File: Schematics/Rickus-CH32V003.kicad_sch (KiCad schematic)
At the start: 31 parts, among them J1 USB_C_Receptacle_USB2.0, J3 Conn_01x03, J4 OledDisplay, J6 uSD Card, SW2 Power, SW2 SW_MEC_5E, U1 CH32V003f4p6, U1 CH340E, U2 8 megabytes SPI PSRAM, U3 LD1117S12TR_SOT223

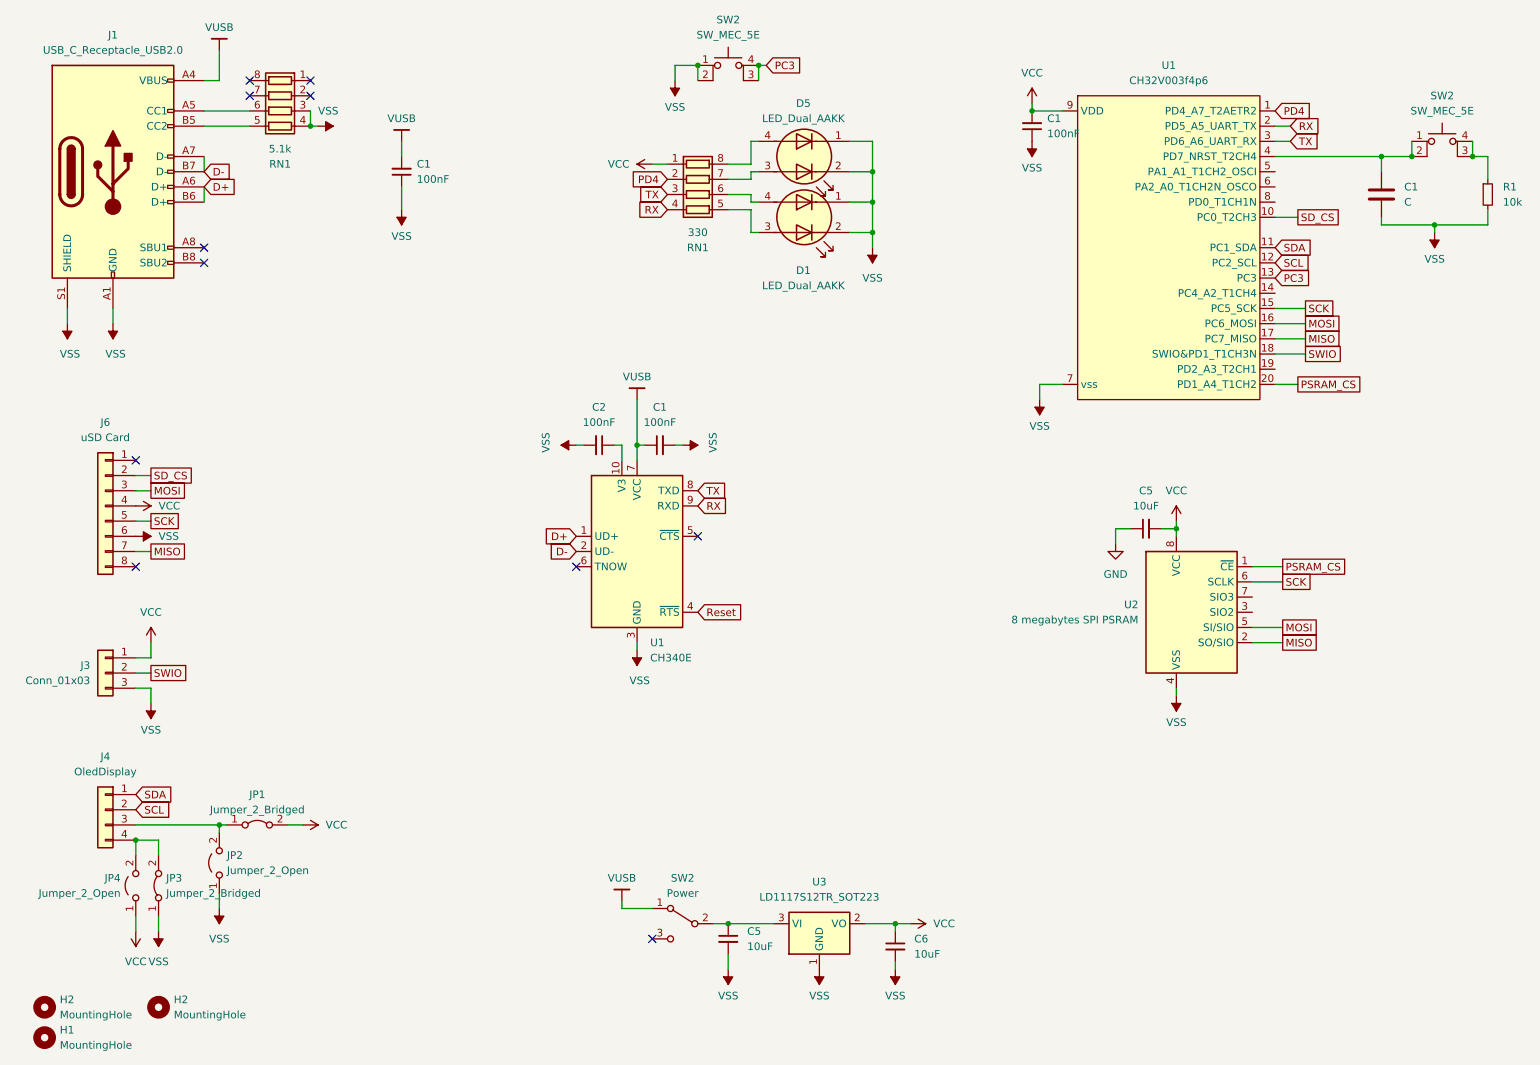
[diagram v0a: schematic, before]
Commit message: V1 completed and ordered
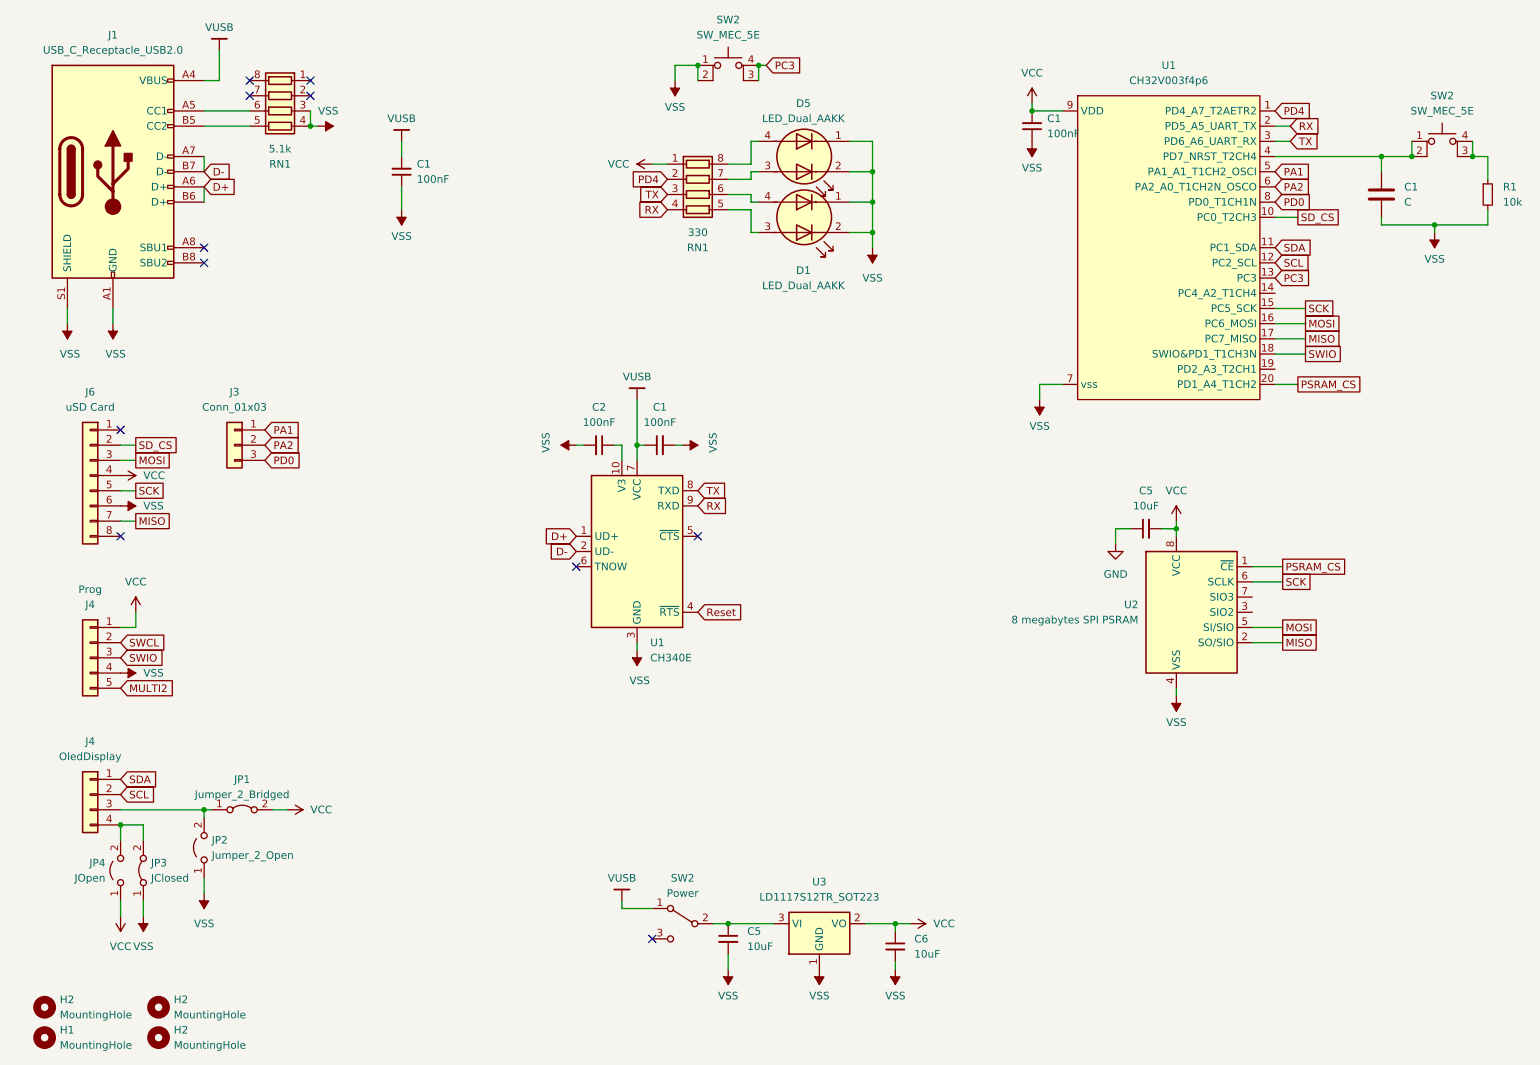
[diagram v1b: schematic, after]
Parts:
- added H2: MountingHole, MountingHole:MountingHole_2.2mm_M2, symbol Mechanical:MountingHole
- added J4: Prog, Connector_PinHeader_2.54mm:PinHeader_1x05_P2.54mm_Vertical, symbol Connector_Generic:Conn_01x05
- JP3: value Jumper_2_Bridged -> JClosed
- JP4: value Jumper_2_Open -> JOpen
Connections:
- net SWIO: now also J4.3 (Pin_3); no longer J3.2 (Pin_2)
- net VCC: now also J4.1 (Pin_1); no longer J3.1 (Pin_1)
- net VSS: now also J4.4 (Pin_4); no longer J3.3 (Pin_3)
- net PA1: now reaches U1.5 (PA1_A1_T1CH2_OSCI)
- net PA1: now also J3.1 (Pin_1)
- net PA2: now reaches U1.6 (PA2_A0_T1CH2N_OSCO)
- net PA2: now also J3.2 (Pin_2)
- net PD0: now reaches U1.8 (PD0_T1CH1N)
- net PD0: now also J3.3 (Pin_3)
- new net MULTI2: J4.5 (Pin_5)
- new net SWCL: J4.2 (Pin_2)
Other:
- moved on the sheet: J4, J6, JP1, JP2, JP3, JP4
